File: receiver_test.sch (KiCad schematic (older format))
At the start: 9 parts, among them J1 Conn_Coaxial, J2 Conn_Coaxial, J3 Conn_01x02_Male, J4 Conn_01x02_Male, J5 Conn_01x02_Male, U1 ADE-1H+

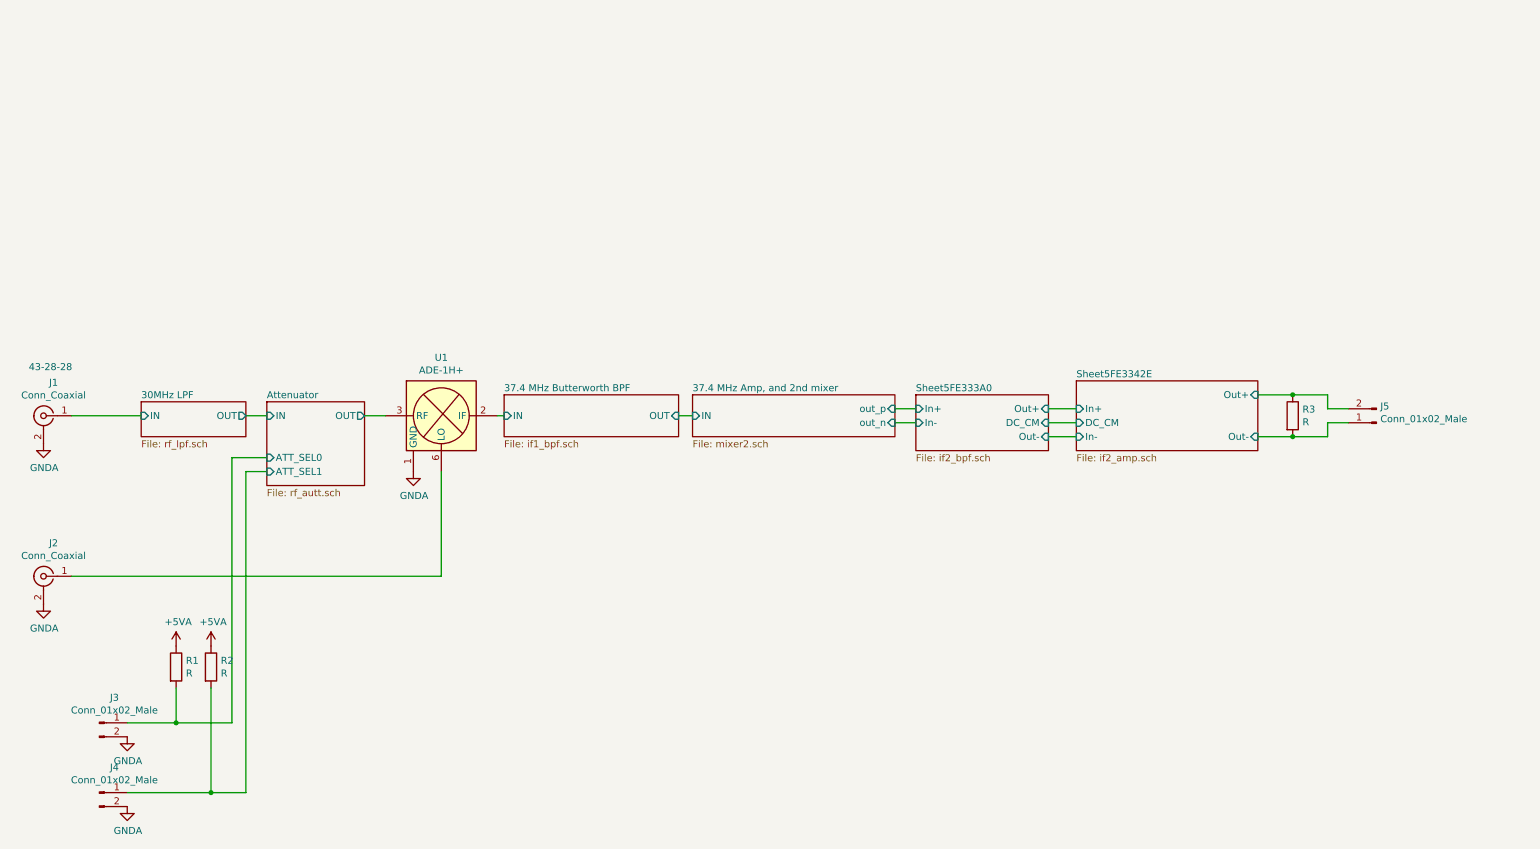
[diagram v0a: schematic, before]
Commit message: Nyáktervezésre majdnem kész
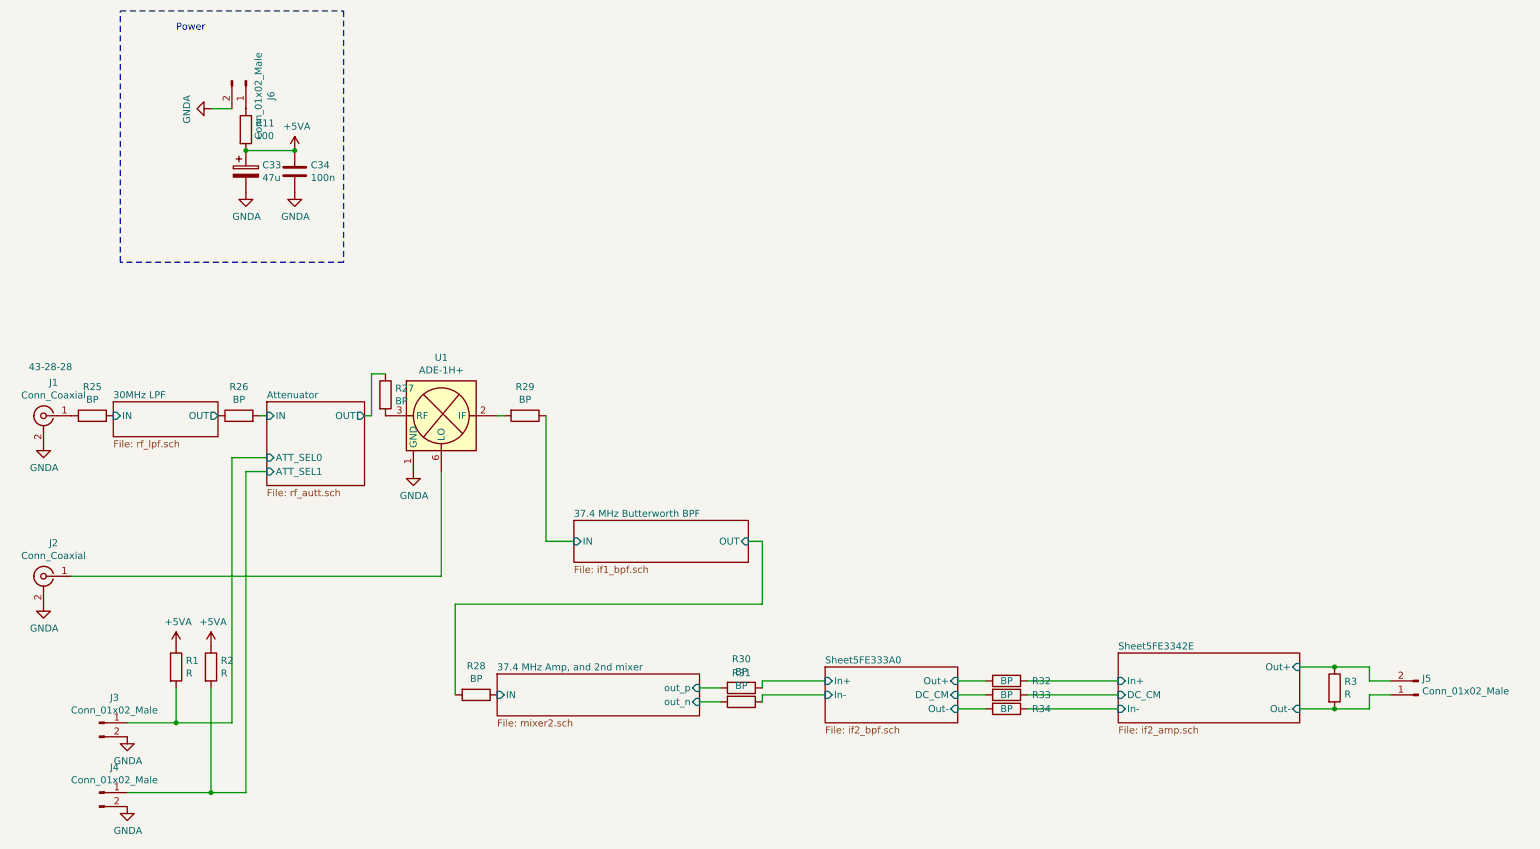
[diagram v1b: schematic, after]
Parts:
- added C33: 47u, Capacitor_SMD:CP_Elec_6.3x5.3, symbol Device:CP
- added C34: 100n, Capacitor_SMD:C_0805_2012Metric_Pad1.15x1.40mm_HandSolder, symbol Device:C
- added J6: Conn_01x02_Male, Connector_PinSocket_2.54mm:PinSocket_1x02_P2.54mm_Vertical, symbol Connector:Conn_01x02_Male
- added R11: 100, Resistor_SMD:R_0805_2012Metric_Pad1.15x1.40mm_HandSolder, symbol Device:R
- added R25, R26, R27, R28, R29, R30, R31, R32, R33, R34: BP, Resistor_SMD:R_1206_3216Metric_Pad1.42x1.75mm_HandSolder, symbol Device:R
- J2: footprint (none) -> Connector_Coaxial:SMA_Molex_73251-1153_EdgeMount_Horizontal
- J3, J4, J5: footprint (none) -> Connector_PinSocket_2.54mm:PinSocket_1x02_P2.54mm_Vertical
- R1, R2, R3: footprint (none) -> Resistor_SMD:R_0805_2012Metric_Pad1.15x1.40mm_HandSolder
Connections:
- net +5VA: now also C33.1, C34.1, R11.2
- net 30MHz LPF/IN: now also R25.2; no longer J1.1 (In)
- net 30MHz LPF/OUT: now also R26.1
- net 37.4 MHz Amp, and 2nd mixer/IN: now also R28.1
- net 37.4 MHz Amp, and 2nd mixer/out_n: now also R31.2
- net 37.4 MHz Amp, and 2nd mixer/out_p: now also R30.2
- net 37.4 MHz Butterworth BPF/IN: now also R29.1; no longer U1.2 (IF)
- net Attenuator/OUT: now also R27.1; no longer U1.3 (RF)
- net GNDA: now also C33.2, C34.2, J6.2 (Pin_2)
- net Sheet5FE333A0/DC_CM: now also R33.2
- net Sheet5FE333A0/Out+: now also R32.2
- net Sheet5FE333A0/Out-: now also R34.2
- new net: J1.1 (In), R25.1
- new net: R29.2, U1.2 (IF)
- new net: R27.2, U1.3 (RF)
- new net: J6.1 (Pin_1), R11.1
- new net 37.4 MHz Butterworth BPF/OUT: R28.2
- new net Attenuator/IN: R26.2
- new net Sheet5FE333A0/In+: R30.1
- new net Sheet5FE333A0/In-: R31.1
- new net Sheet5FE3342E/DC_CM: R33.1
- new net Sheet5FE3342E/In+: R32.1
- new net Sheet5FE3342E/In-: R34.1
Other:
- note added: "Power\n"
- moved on the sheet: J5, R3
